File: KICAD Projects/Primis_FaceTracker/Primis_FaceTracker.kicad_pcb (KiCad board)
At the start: 2 copper layers, 47 parts, among them CN2 KH-FG0.5-H2.0-24PIN, J1 USB_C_Receptacle_USB2.0_16P, Q1 PMOS, SW1 SW_SPST, SW2 SW_SPST, U1 ESP32-S3-WROOM-1, U2 AMS1117-3.3, U3 XC6206P122MR, U5 XC6206P282MR

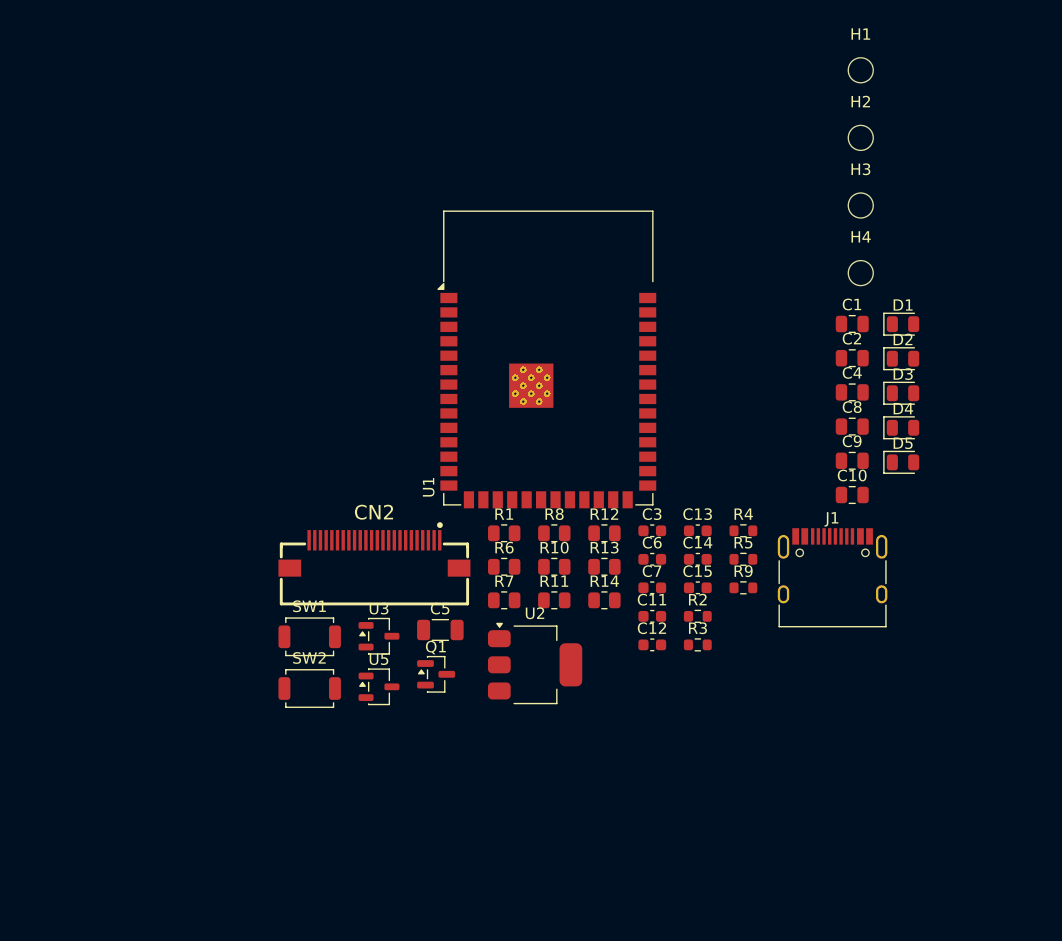
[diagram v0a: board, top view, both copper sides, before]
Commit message: Face Tracker PCB
-Some work on the PCB, not quite done but I'm making some changes so uploading as a backup.
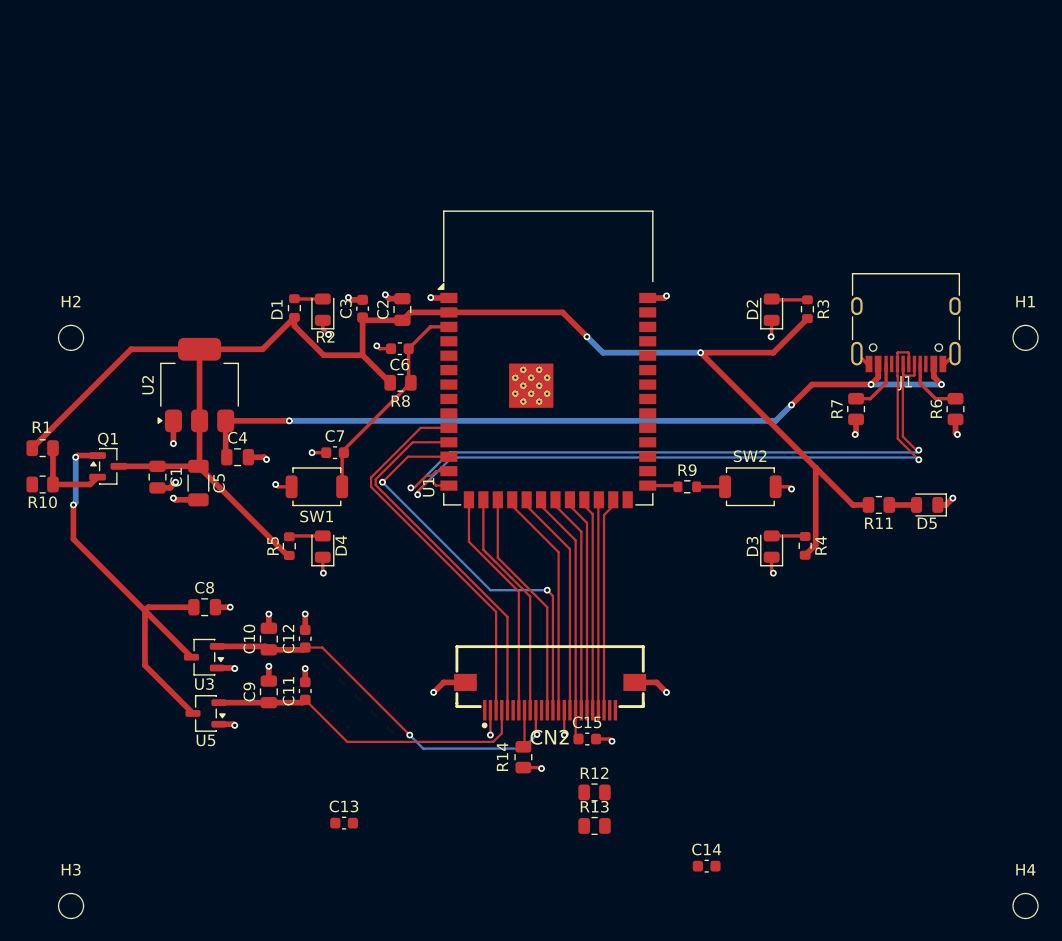
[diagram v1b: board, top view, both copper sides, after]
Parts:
- moved H3 92.9 mm to (120.6, 129.3)
- moved H2 71.7 mm to (120.6, 79.3)
- moved C1 62.6 mm to (128.2, 91.5), turned to -90 degrees
- moved C8 59.2 mm to (132.3, 103.0)
- moved H4 57.6 mm to (204.6, 129.3)
- moved C9 55.2 mm to (138.0, 110.5), turned to 90 degrees
- moved C4 54.4 mm to (135.2, 89.8)
- moved C10 52.9 mm to (138.0, 105.8), turned to 90 degrees
- moved D4 52.1 mm to (142.8, 97.7), turned to 90 degrees
- moved D1 51.1 mm to (142.8, 76.8), turned to 90 degrees
- moved R10 45.6 mm to (118.1, 92.2)
- moved R2 44.7 mm to (140.2, 76.7), turned to -90 degrees
- moved SW2 42.7 mm to (180.4, 92.4)
- moved R6 42.1 mm to (198.4, 85.6), turned to 90 degrees
- moved R1 41.3 mm to (118.1, 89.0), turned to 180 degrees
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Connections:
- net Net-(U1-USB_D+) renamed D+
- net Net-(U1-USB_D-) renamed D-
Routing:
- net CAM_RST: track 0.00 -> 141.7 mm, vias 0 -> 2
- net +5V: track 0.00 -> 71.7 mm, vias 0 -> 4
- net D+: track 0.00 -> 61.5 mm, vias 0 -> 2
- net D-: track 0.00 -> 61.3 mm, vias 0 -> 2
- net GND: track 0.00 -> 55.9 mm, vias 0 -> 32
- net Net-(Q1-D): track 0.00 -> 39.2 mm, vias 0 -> 2
- net CAM_MCLK: track 0.00 -> 36.0 mm, vias 0 -> 2
- net CAM_1.2V: track 0.00 -> 34.7 mm, vias 0 -> 2
- net CAM_SDA: track 0.00 -> 33.7 mm
- net CAM_SCK: track 0.00 -> 32.9 mm
- net CAM_2.8V: track 0.00 -> 28.9 mm
- net CAM_PCLK: track 0.00 -> 22.4 mm
- net CAM_VSYNC: track 0.00 -> 20.3 mm
- net CAM_D7: track 0.00 -> 20.3 mm
- net CAM_HSYNC: track 0.00 -> 20.2 mm
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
